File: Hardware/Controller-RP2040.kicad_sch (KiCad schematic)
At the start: 43 parts, among them J1 Conn_01x07_Male, J2 Conn_01x04_Male, J3 Conn_01x02_Male, J4 Conn_01x02_Male, J5 Conn_01x02_Male, J6 Conn_01x02_Male, J7 Conn_01x08_Male, J8 QWIIC_Vertical, J9 QWIIC_Stackable, Q1 DMG1012T, U1 RP2040, U2 W25Q32JVXGIQ, Y1 12MHz

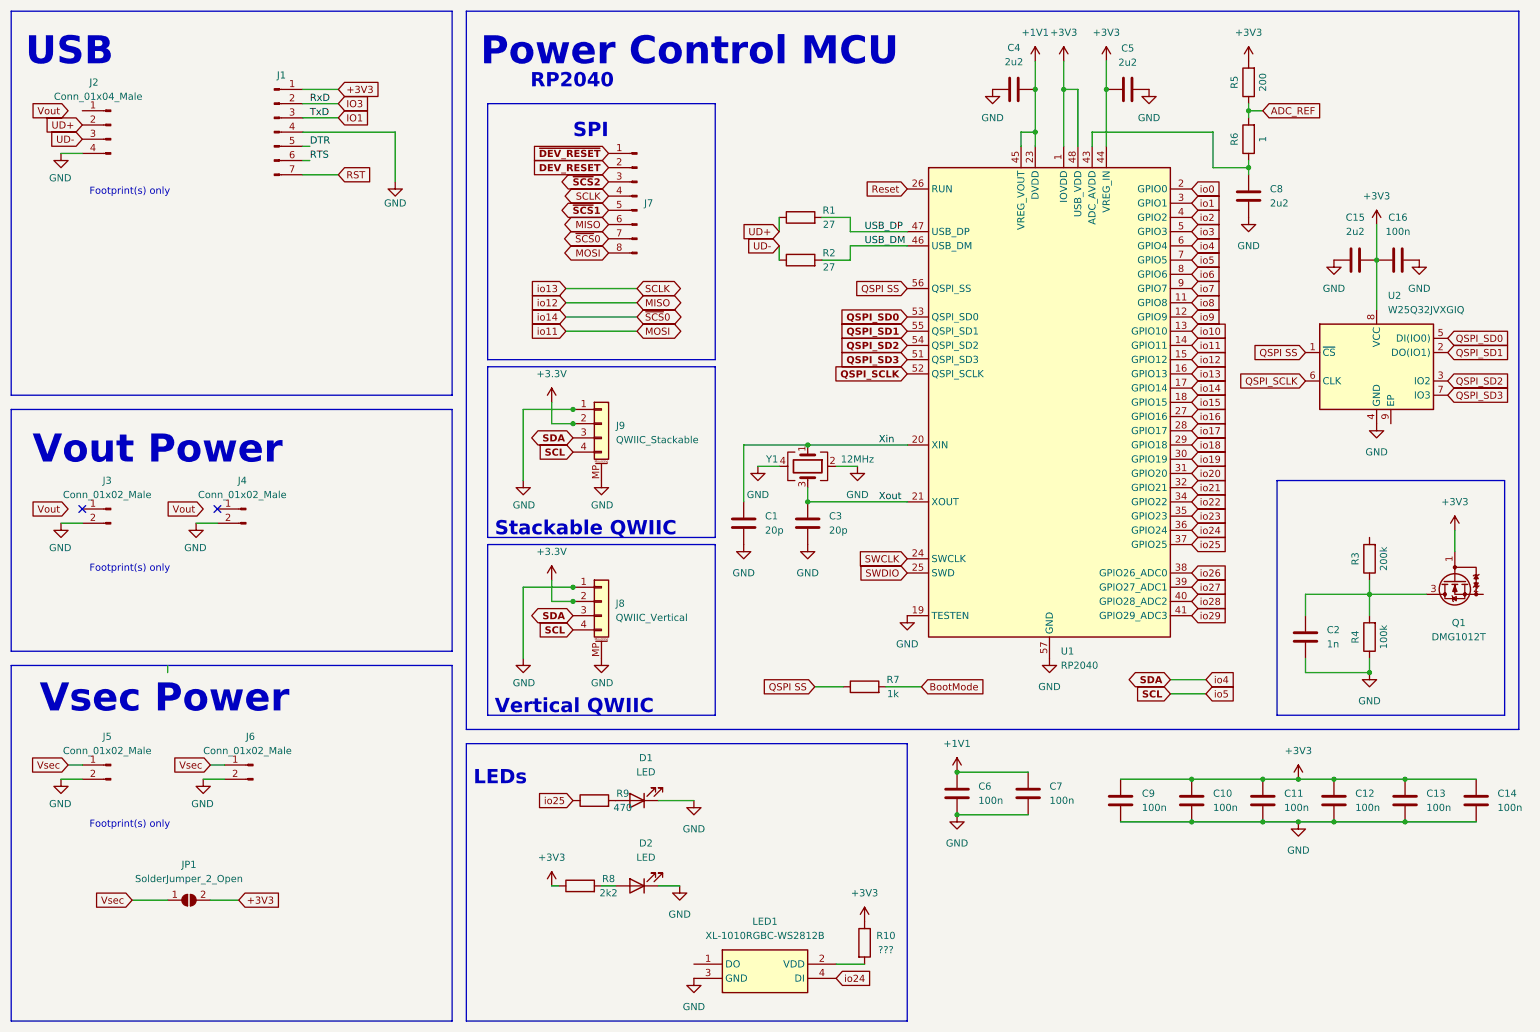
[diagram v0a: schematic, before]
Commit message: Working on the RP2040 & cleaning up stuff...
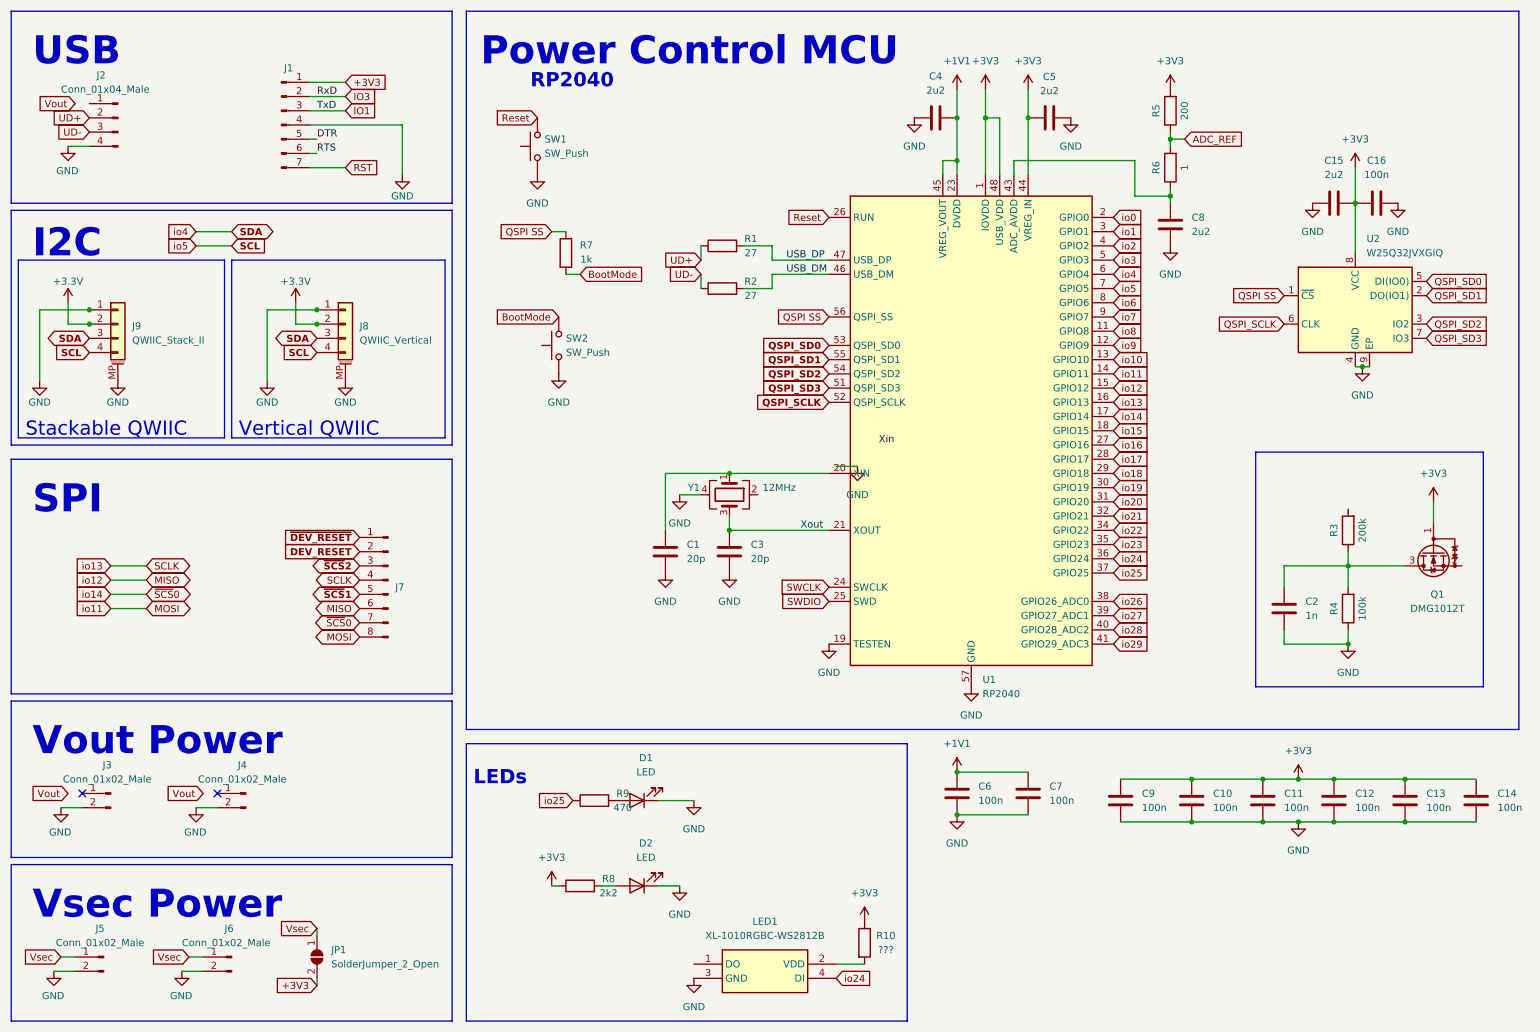
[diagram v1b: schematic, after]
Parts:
- added SW1, SW2: SW_Push, Tinker:SW_Push_TS273014TP, symbol Switch:SW_Push
- J9: value QWIIC_Stackable -> QWIIC_Stack_II
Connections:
- net BootMode: now also SW2.2
- net GND: now also U2.9 (EP), SW1.1, SW2.1; no longer Y1.2
- net Reset: now also SW1.2
- net Xin: no longer C1.1, U1.20 (XIN), Y1.1
- new net: C1.1, U1.20 (XIN), Y1.1
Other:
- note added: "I2C"
- note removed: "Footprint(s) only"
- moved on the sheet: C1, C15, C16, C2, C3, C4, C5, C8, J1, J2, J3, J4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
